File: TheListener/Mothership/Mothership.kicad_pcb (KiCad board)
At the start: 2 copper layers, 81 parts, among them J1 RJ45, J2 RJ45, J3 RJ45, J4 RJ45, J5 RJ45, J6 RJ45, J7 RJ45, J8 RJ45, J9 Conn_01x02_Female, U1 SP3491, U10 AMS1117-3.3, U11 NID35-5, U12 Teensy3.5, U2 SP3491, U3 SP3491, U4 SP3491, U5 SP3491, U6 SP3491, U7 SP3491, U8 SP3491, U9 AMS1117-3.3

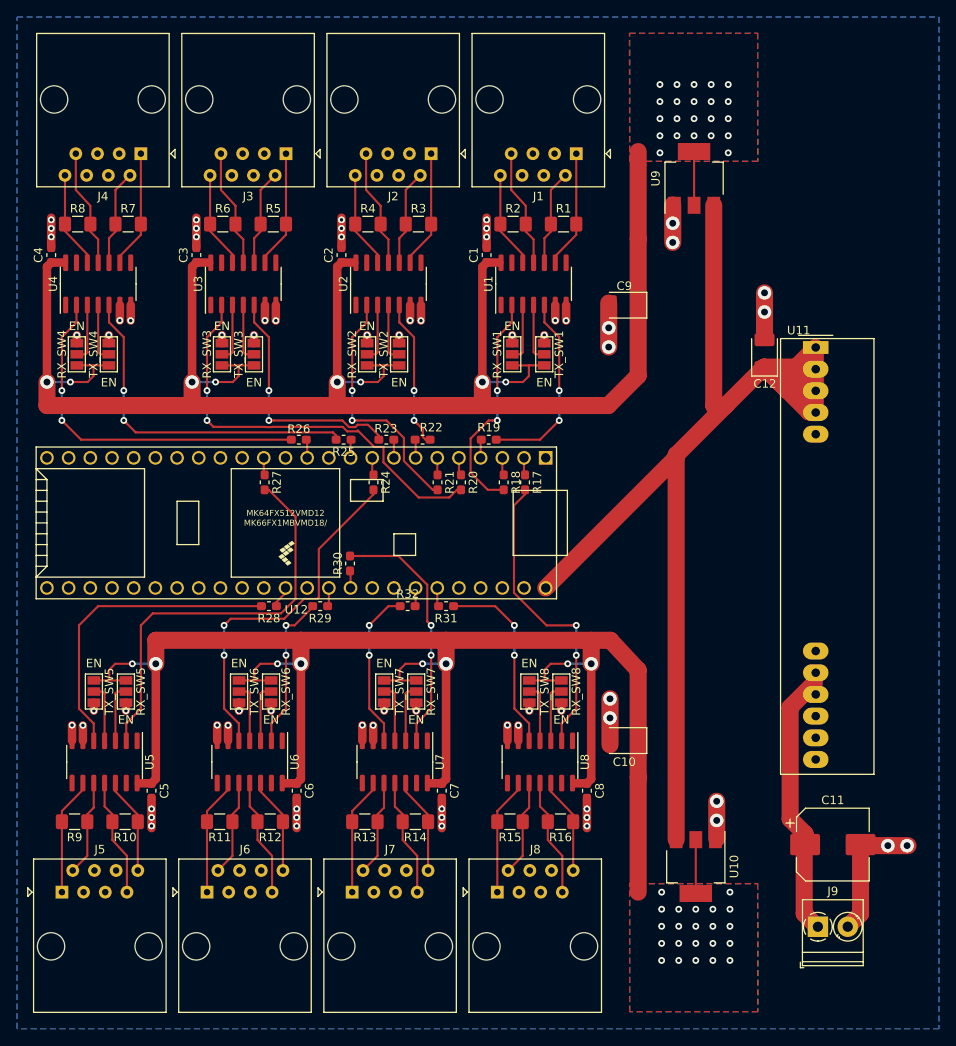
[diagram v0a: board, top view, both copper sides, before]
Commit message: updates
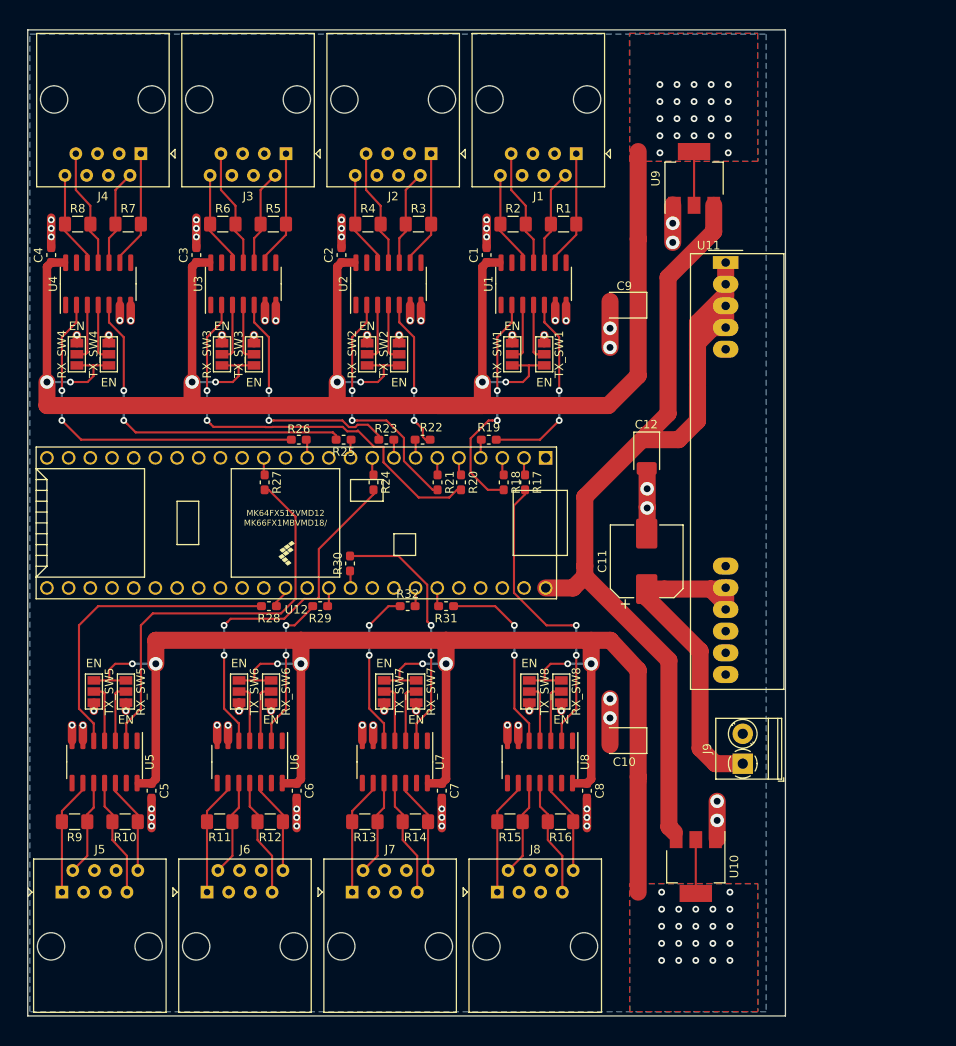
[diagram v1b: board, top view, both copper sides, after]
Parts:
- moved C11 39.7 mm to (117.8, 83.8), turned to 90 degrees
- moved J9 21.0 mm to (129.0, 107.5), turned to 90 degrees
- moved C12 18.2 mm to (117.8, 71.2), turned to 270 degrees
- moved U11 14.5 mm to (127.0, 48.8)
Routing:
- net +5V: track 146.5 -> 128.5 mm
- net GND: track 112.6 -> 99.2 mm, vias 69 -> 67
- net +24V: track 31.1 -> 41.5 mm
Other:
- board outline added: 88.8 x 115.5 mm
